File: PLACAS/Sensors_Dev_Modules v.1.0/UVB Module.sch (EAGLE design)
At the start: 5 parts

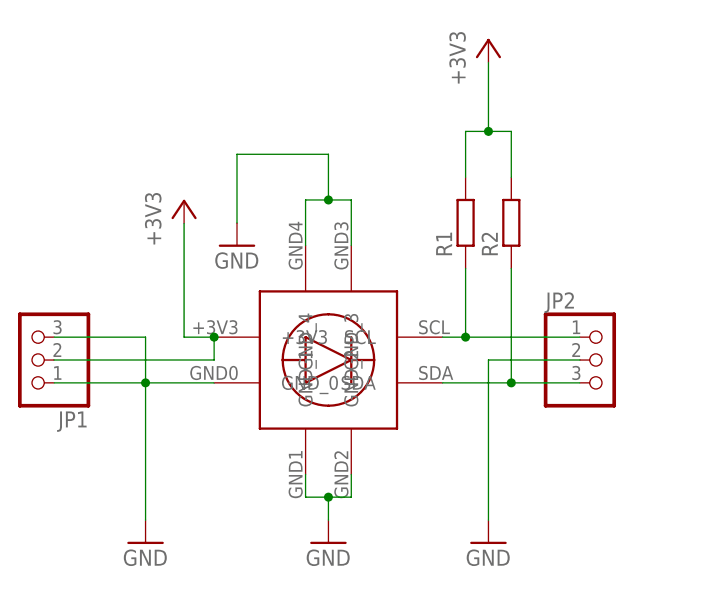
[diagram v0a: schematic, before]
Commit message: Add files via upload
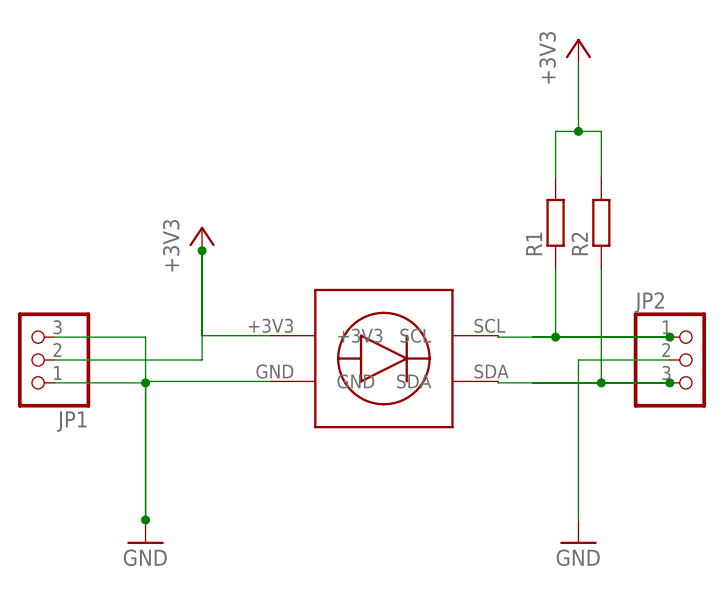
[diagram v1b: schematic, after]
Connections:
- net GND: now also U$1.GND; no longer U$1.GND_0, U$1.GND_1, U$1.GND_2, U$1.GND_3, U$1.GND_4
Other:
- moved on the sheet: JP2, R1, R2
